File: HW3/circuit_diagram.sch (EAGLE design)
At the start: 17 parts

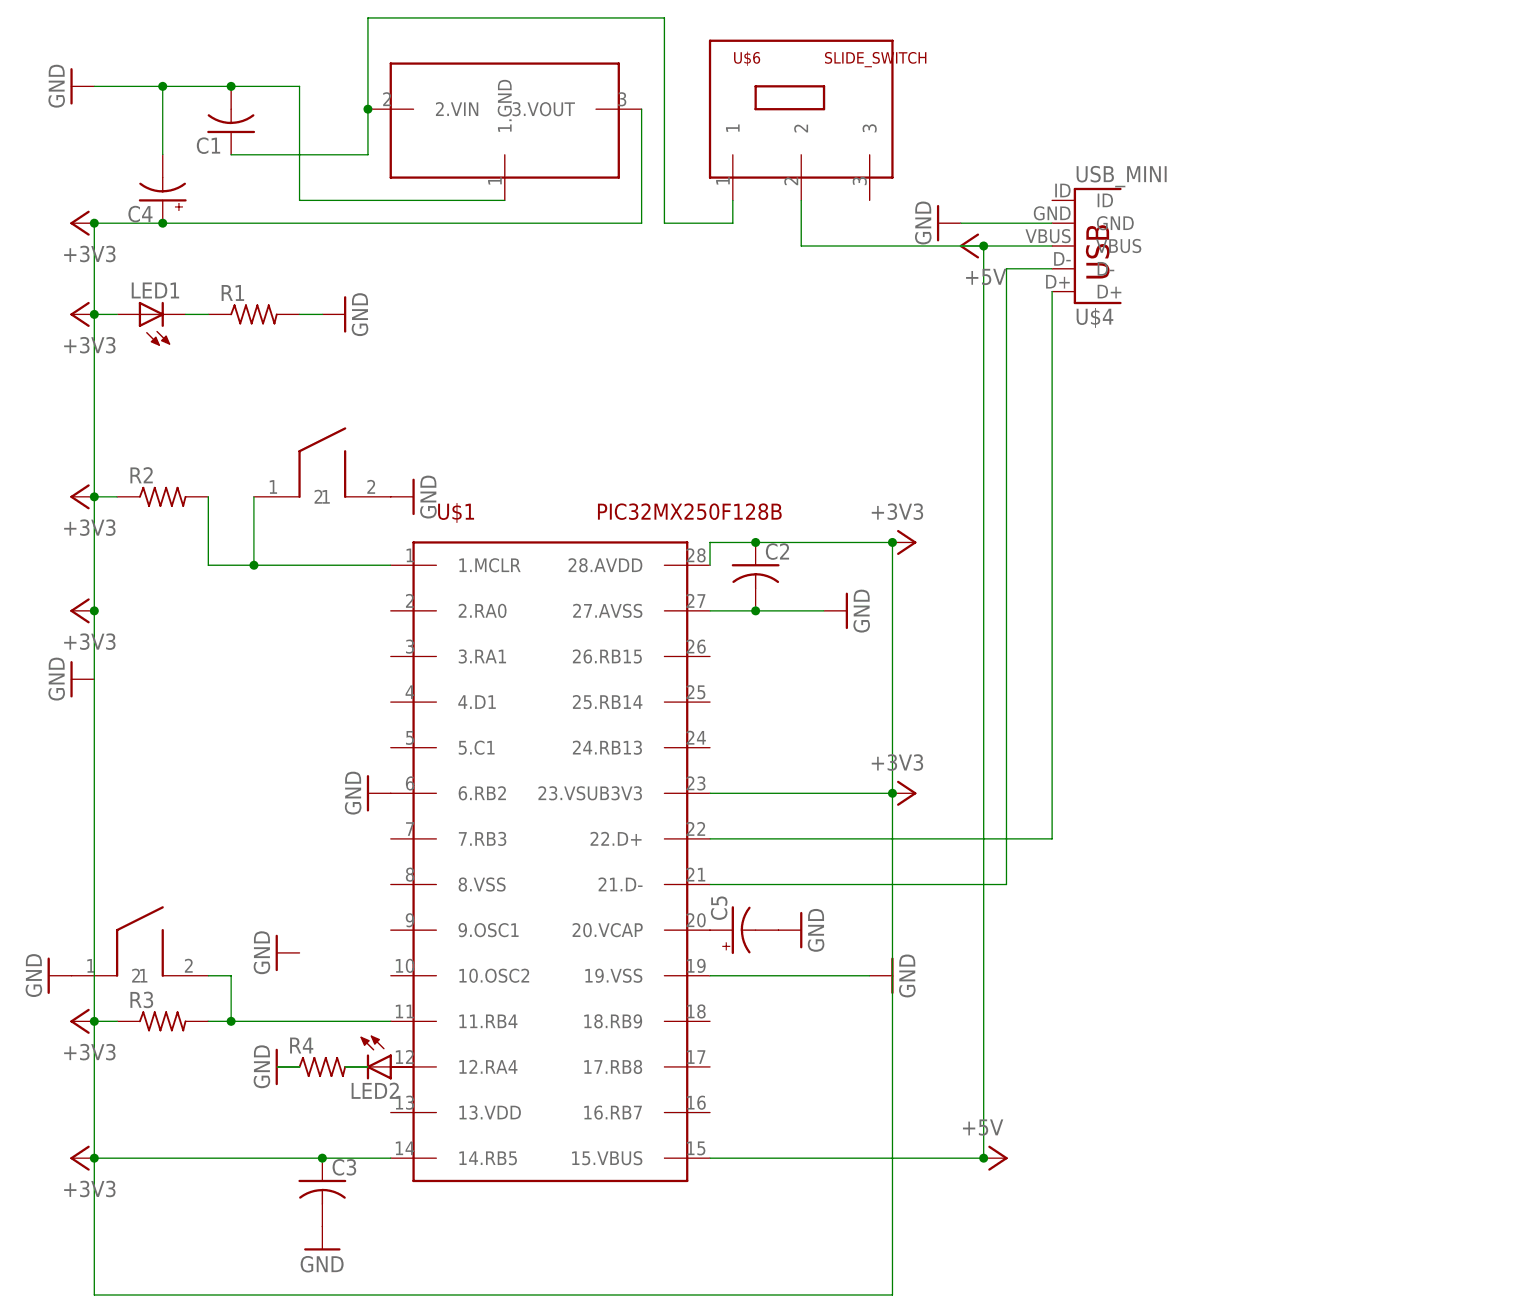
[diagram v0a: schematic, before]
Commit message: Finished schematic
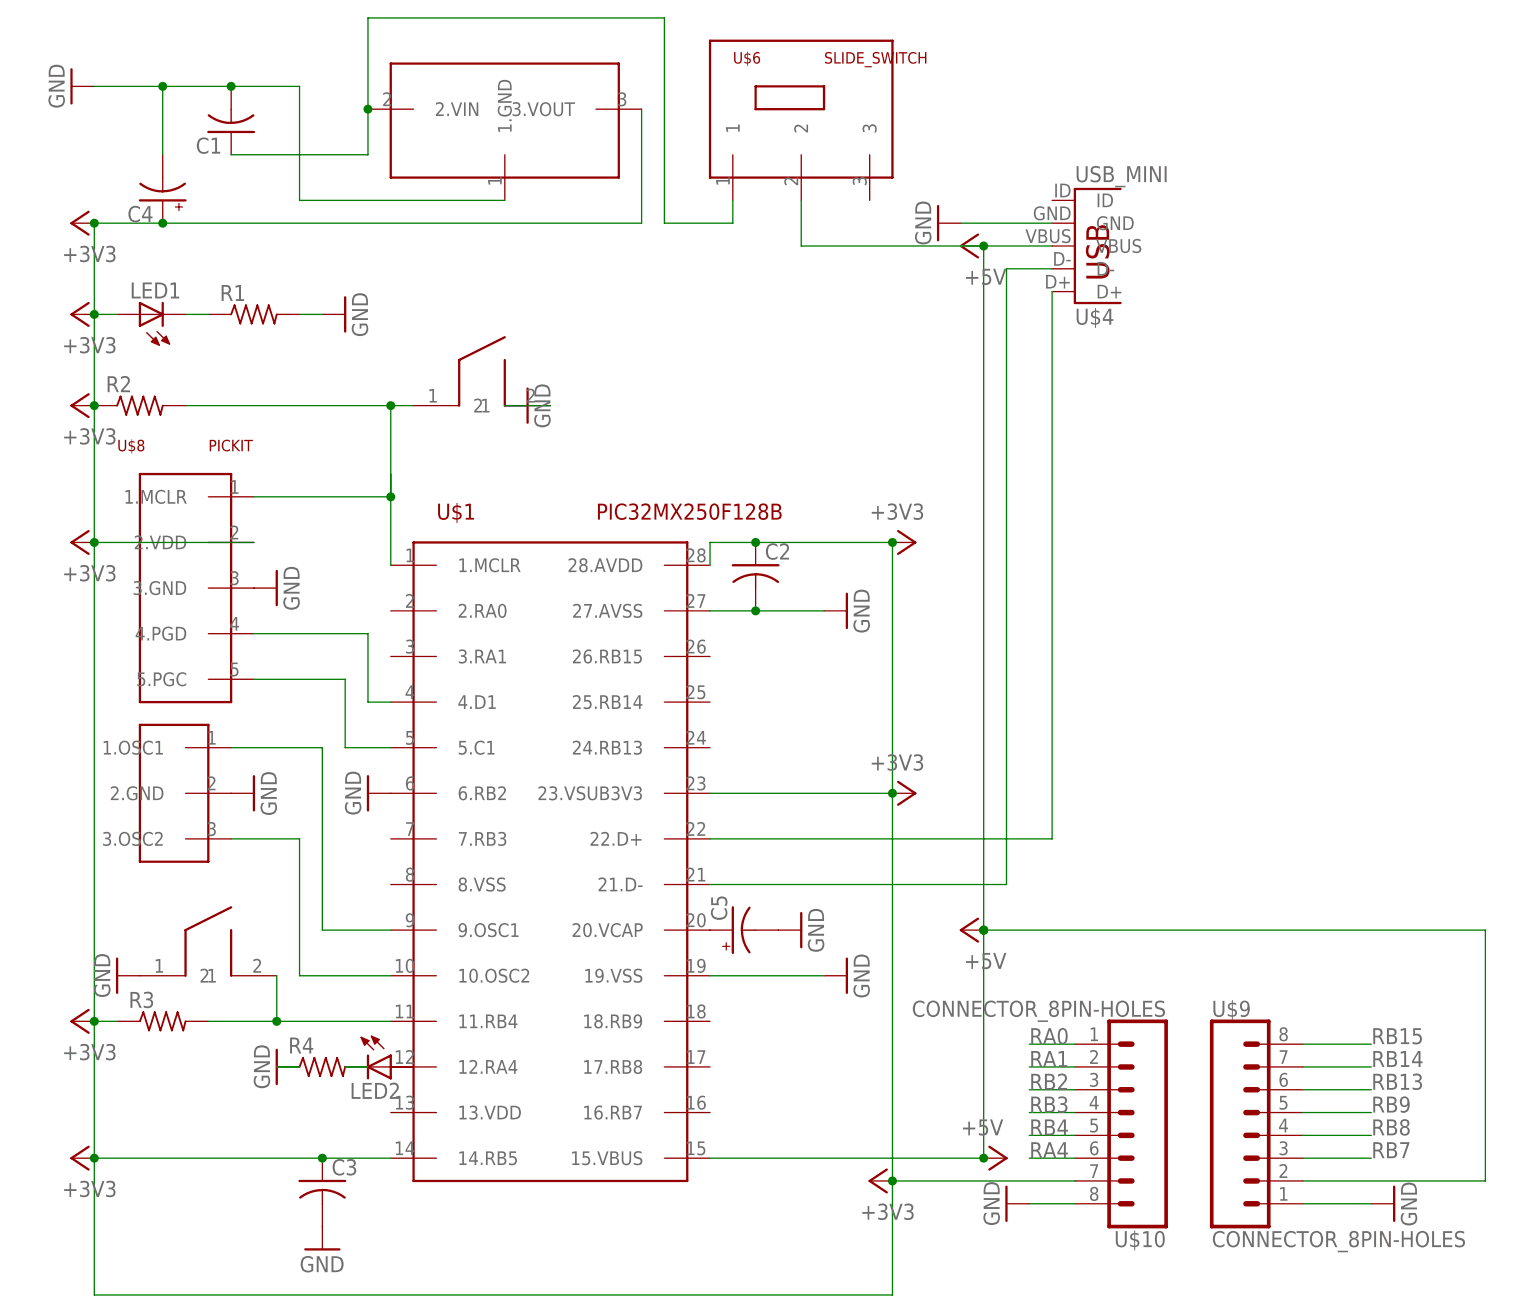
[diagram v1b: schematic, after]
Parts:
- added U$10, U$9: CONNECTOR_8PIN-HOLES, connectior-8pin-holes:CONNECTOR_8PIN-HOLES
- added U$7: OSC, OSC:OSC
- added U$8: PICKIT, pickit:PICKIT
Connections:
- new net N$10: U$1.10.OSC2, U$7.3.OSC2
- new net N$11: U$1.5.C1, U$8.5.PGC
- new net N$12: U$1.4.D1, U$8.4.PGD
- new net N$9: U$1.9.OSC1, U$7.1.OSC1
- new net RA0: U$10.1
- new net RA1: U$10.2
- new net RA4: U$10.6
- new net RB13: U$9.6
- new net RB14: U$9.7
- new net RB15: U$9.8
- new net RB2: U$10.3
- new net RB3: U$10.4
- new net RB4: U$10.5
- new net RB7: U$9.3
- new net RB8: U$9.4
- new net RB9: U$9.5
- net +3V3: now also U$10.7, U$8.2.VDD
- net +5V: now also U$9.2
- net GND: now also U$10.8, U$7.2.GND, U$8.3.GND, U$9.1
- net N$3: now also U$8.1.MCLR
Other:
- moved on the sheet: R2
